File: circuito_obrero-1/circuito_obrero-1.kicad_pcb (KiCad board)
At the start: 2 copper layers, 112 x 98.5 mm, 60 parts, among them U1 74HC165, U2 74HC165

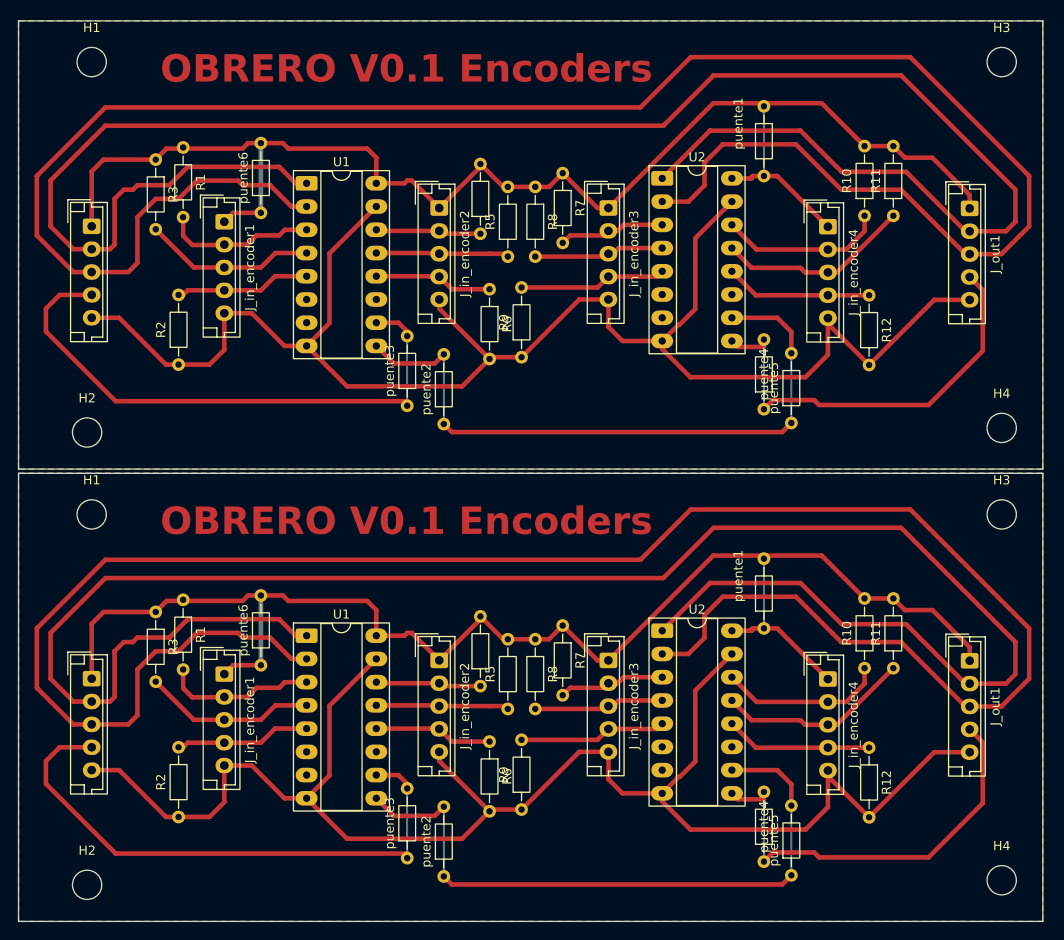
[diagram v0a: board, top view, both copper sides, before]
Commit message: ajustes en en circuito
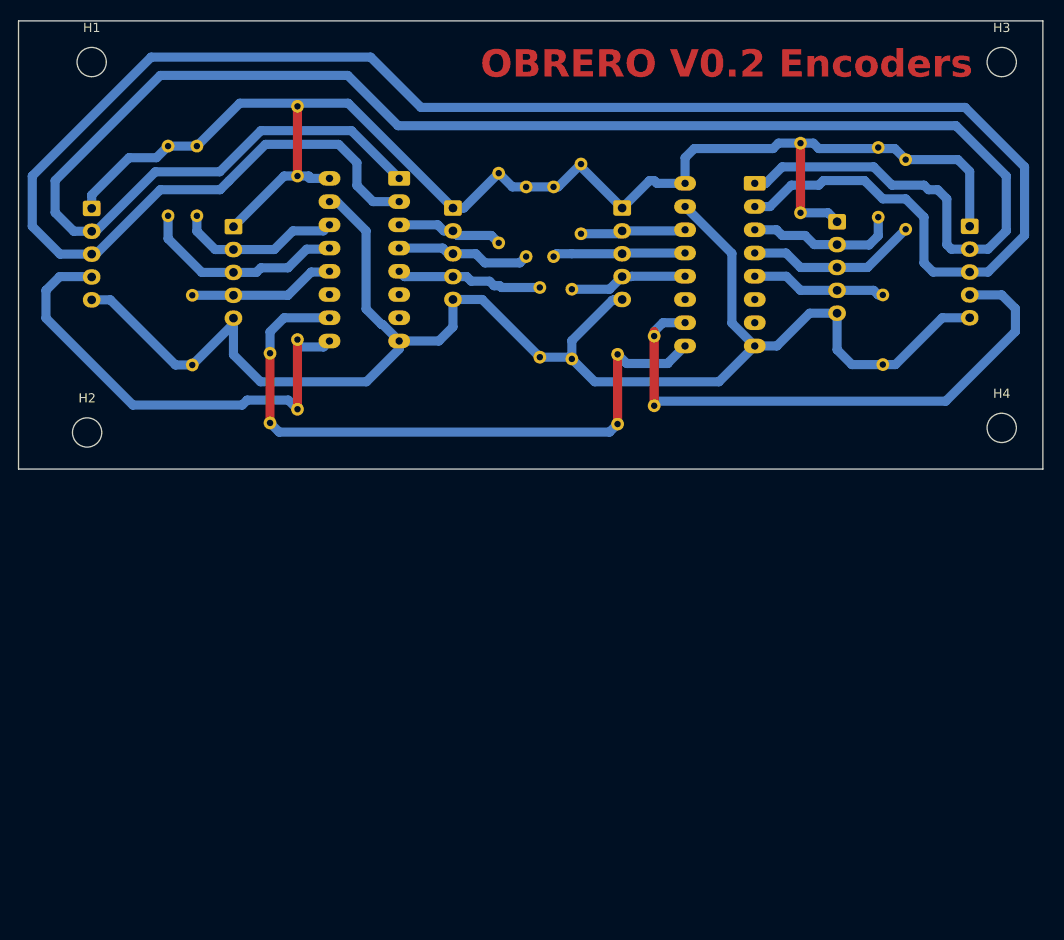
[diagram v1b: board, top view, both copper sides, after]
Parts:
- removed the H1 at (97.0, 79.5)
- removed the H2 at (96.5, 120.0)
- removed the H3 at (196.5, 79.5)
- removed the H4 at (196.5, 119.5)
- removed the J_in1 at (97.0, 97.5)
- removed the J_in_encoder1 at (111.5, 97.0)
- removed the J_in_encoder2 at (135.0, 95.5)
- removed the J_in_encoder3 at (153.5, 95.5)
- removed the J_in_encoder4 at (177.5, 97.5)
- removed the J_out1 at (193.0, 95.5)
- removed the R1 at (107.0, 88.8)
- removed the R10 at (181.5, 96.3)
- removed the R11 at (184.7, 96.3)
- removed the R12 at (182.0, 105.0)
- removed the R2 at (106.5, 112.6)
- removed the R3 at (104.0, 90.2)
- removed the R4 at (139.5, 98.3)
- removed the R5 at (142.5, 100.8)
- removed the R6 at (140.5, 104.3)
- removed the R7 at (148.5, 91.7)
- removed the R8 at (145.5, 93.2)
- removed the R9 at (144.0, 111.8)
- removed the U1 at (120.5, 92.8)
- removed the U2 at (159.4, 92.2)
- removed the puente1 at (170.5, 92.0)
- removed the puente2 at (135.5, 119.1)
- removed the puente3 at (131.5, 117.1)
- removed the puente4 at (170.5, 117.5)
- removed the puente5 at (173.5, 119.0)
- removed the puente6 at (115.5, 96.0)
- J_in1, J_in_encoder1, J_in_encoder2, J_in_encoder3, J_in_encoder4, J_out1, R1, R10, R11, R12, R2, R3, R4, R5, R6, R7, R8, R9, U1, U2, puente1, puente2, puente3, puente4, puente5, puente6: moved to B.Cu
- moved J_in1 96.0 mm to (193.0, 48.0)
- moved J_out1 96.0 mm to (97.0, 46.0)
- moved R3 82.0 mm to (186.0, 40.7)
- moved R11 79.3 mm to (105.3, 46.9)
- moved R2 77.0 mm to (183.5, 63.1)
- moved R1 76.0 mm to (183.0, 39.4)
- moved R12 74.0 mm to (108.0, 55.5)
- moved R10 73.0 mm to (108.5, 46.9)
- moved J_in_encoder1 67.0 mm to (178.5, 47.5)
- moved J_in_encoder4 65.0 mm to (112.5, 48.0)
- moved puente6 59.0 mm to (174.5, 46.5)
- moved puente5 57.0 mm to (116.5, 69.5)
- moved puente1 51.0 mm to (119.5, 42.5)
- moved puente4 51.0 mm to (119.5, 68.0)
- moved U1 49.0 mm to (169.5, 43.3), turned to 180 degrees
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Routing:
- net Net-(J_in1-Pin_3): track 442.2 -> 221.7 mm
- net Net-(J_in1-Pin_2): track 412.3 -> 203.7 mm
- net GND: track 343.9 -> 173.0 mm
- net VCC: track 313.3 -> 156.6 mm
- net Net-(U1-Q7): track 142.9 -> 71.5 mm
- net Net-(J_in1-Pin_4): track 124.4 -> 62.2 mm
- net Net-(J_out1-Pin_4): track 94.1 -> 52.1 mm
- net Net-(J_in_encoder4-Pin_3): track 42.6 -> 22.8 mm
- net Net-(J_in_encoder1-Pin_3): track 37.8 -> 18.9 mm
- net Net-(J_in_encoder4-Pin_2): track 36.3 -> 18.1 mm
- net Net-(J_in_encoder1-Pin_2): track 33.3 -> 16.6 mm
- net Net-(J_in_encoder3-Pin_4): track 32.2 -> 16.1 mm
- net Net-(J_in_encoder4-Pin_4): track 32.2 -> 16.1 mm
- net Net-(J_in_encoder1-Pin_4): track 29.7 -> 14.8 mm
- net Net-(J_in_encoder2-Pin_3): track 29.1 -> 14.5 mm
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- removed copper zone on F.Cu, net GND
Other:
- board size 112 x 98.5 mm -> 112 x 49 mm
- board text added: "OBRERO V0.2 Encoders"
- board text removed: "OBRERO V0.1 Encoders"
